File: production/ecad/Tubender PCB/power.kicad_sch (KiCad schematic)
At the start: 24 parts, among them Q1 CSD19502Q5B, Q2 CSD19502Q5B, U1 LMR36520FADDAR, U2 LM5146RGYR

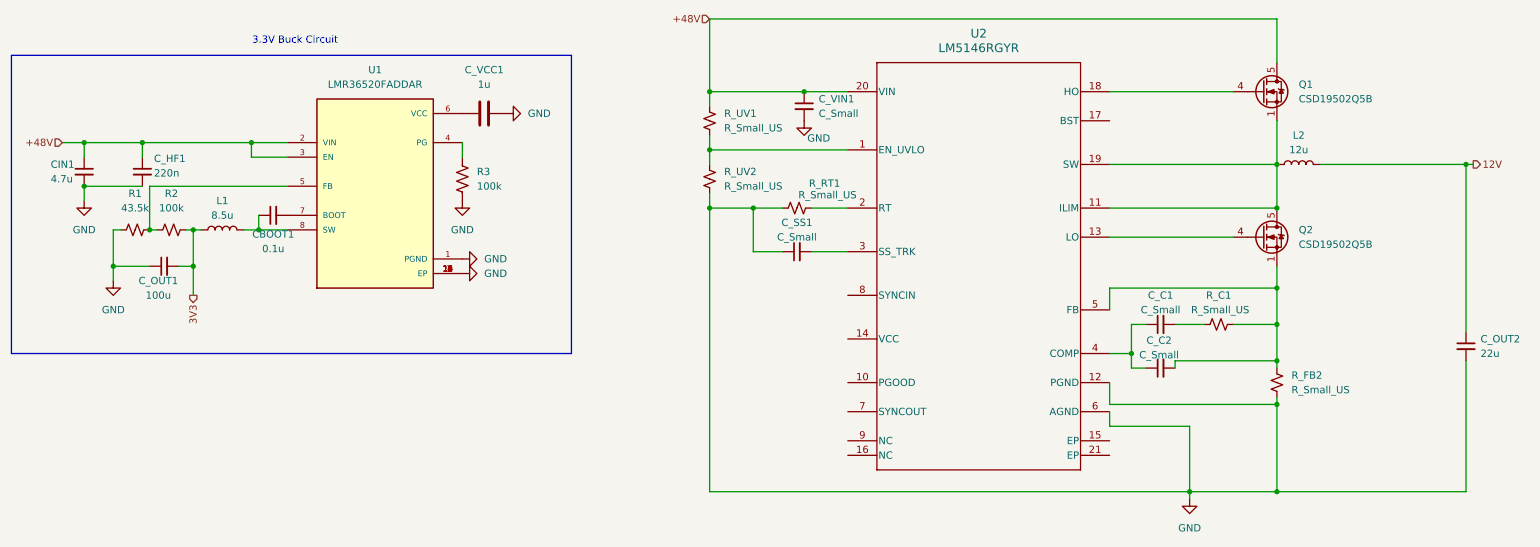
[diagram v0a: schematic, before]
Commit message: All passives valued for 12V buck
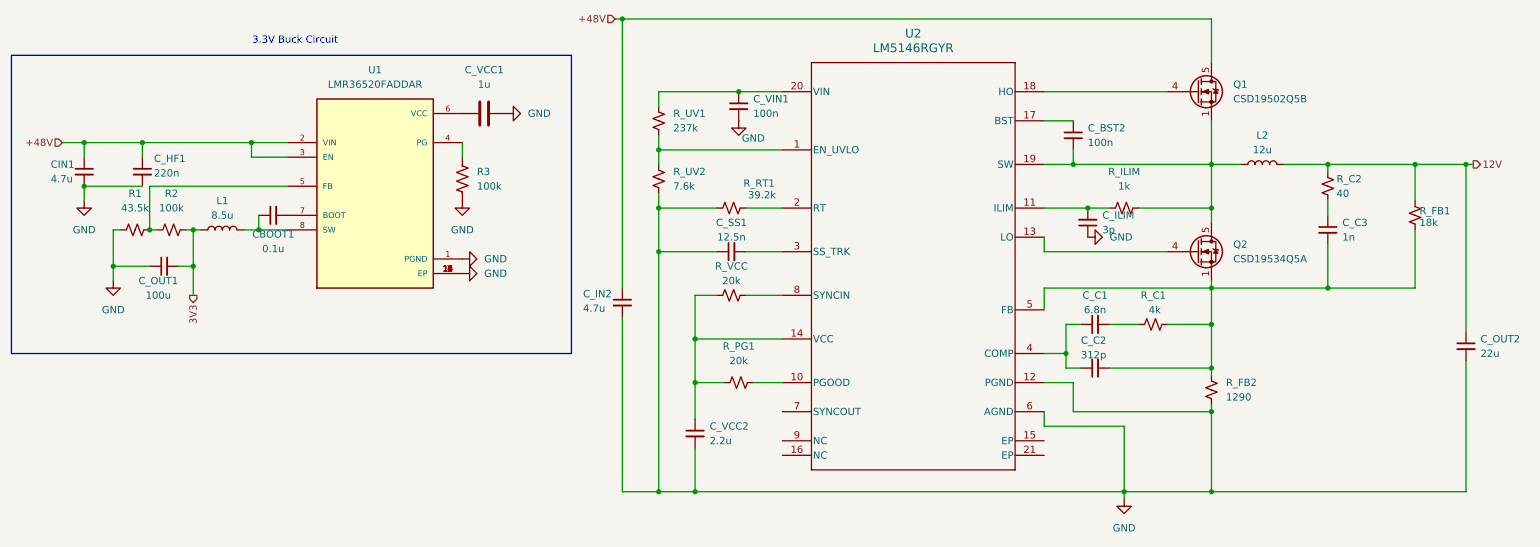
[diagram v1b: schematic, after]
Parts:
- removed Q2: CSD19502Q5B, Package_TO_SOT_SMD:TDSON-8-1, symbol Transistor_FET:CSD19502Q5B
- added C_BST2: 100n, symbol Device:C_Small
- added C_C3: 1n, symbol Device:C_Small
- added C_ILIM: 3p, symbol Device:C_Small
- added C_IN2: 4.7u, symbol Device:C_Small
- added C_VCC2: 2.2u, symbol Device:C_Small
- added Q2: CSD19534Q5A, Package_TO_SOT_SMD:TDSON-8-1, symbol Transistor_FET:CSD19534Q5A
- added R_C2: 40, symbol Device:R_Small_US
- added R_FB1: 18k, symbol Device:R_Small_US
- added R_ILIM: 1k, symbol Device:R_Small_US
- added R_PG1, R_VCC: 20k, symbol Device:R_Small_US
- C_C1: value C_Small -> 6.8n
- C_C2: value C_Small -> 312p
- C_SS1: value C_Small -> 12.5n
- C_VIN1: value C_Small -> 100n
- R_C1: value R_Small_US -> 4k
- R_FB2: value R_Small_US -> 1290
- R_RT1: value R_Small_US -> 39.2k
- R_UV1: value R_Small_US -> 237k
- R_UV2: value R_Small_US -> 7.6k
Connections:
- net +48V: now also C_IN2.1; no longer C_VIN1.1, R_UV1.1, U2.20 (VIN)
- net 12V: now also R_C2.1, R_FB1.1
- net GND: now also C_ILIM.1, C_IN2.2, C_VCC2.2
- net at L2.1, Q1.1 (S), Q1.2 (S)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: now also C_BST2.2, Q2.5 (D), R_ILIM.2; no longer U2.11 (ILIM)
- net at U2.10 (PGOOD): now also R_PG1.2
- net at U2.13 (LO): now also Q2.4 (G)
- net at U2.14 (VCC): now also C_VCC2.1, R_PG1.1, R_VCC.2
- net at U2.17 (BST): now also C_BST2.1
- net at C_C2.2, R_C1.2, R_FB2.1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: now also C_C3.2, Q2.1 (S), Q2.2 (S), Q2.3 (S), R_FB1.2
- net at U2.8 (SYNCIN): now also R_VCC.1
- new net: C_ILIM.2, R_ILIM.1, U2.11 (ILIM)
- new net: C_VIN1.1, R_UV1.1, U2.20 (VIN)
- new net: C_C3.1, R_C2.2
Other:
- moved on the sheet: C_C1, C_C2, C_SS1, C_VIN1, L2, Q1, R_C1, R_FB2, R_RT1, R_UV1, R_UV2, U2
